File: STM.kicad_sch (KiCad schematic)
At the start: 25 parts, among them J7 PIN HEADER 2.54MM PITCH STR D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, U1 STM32L433CCU6

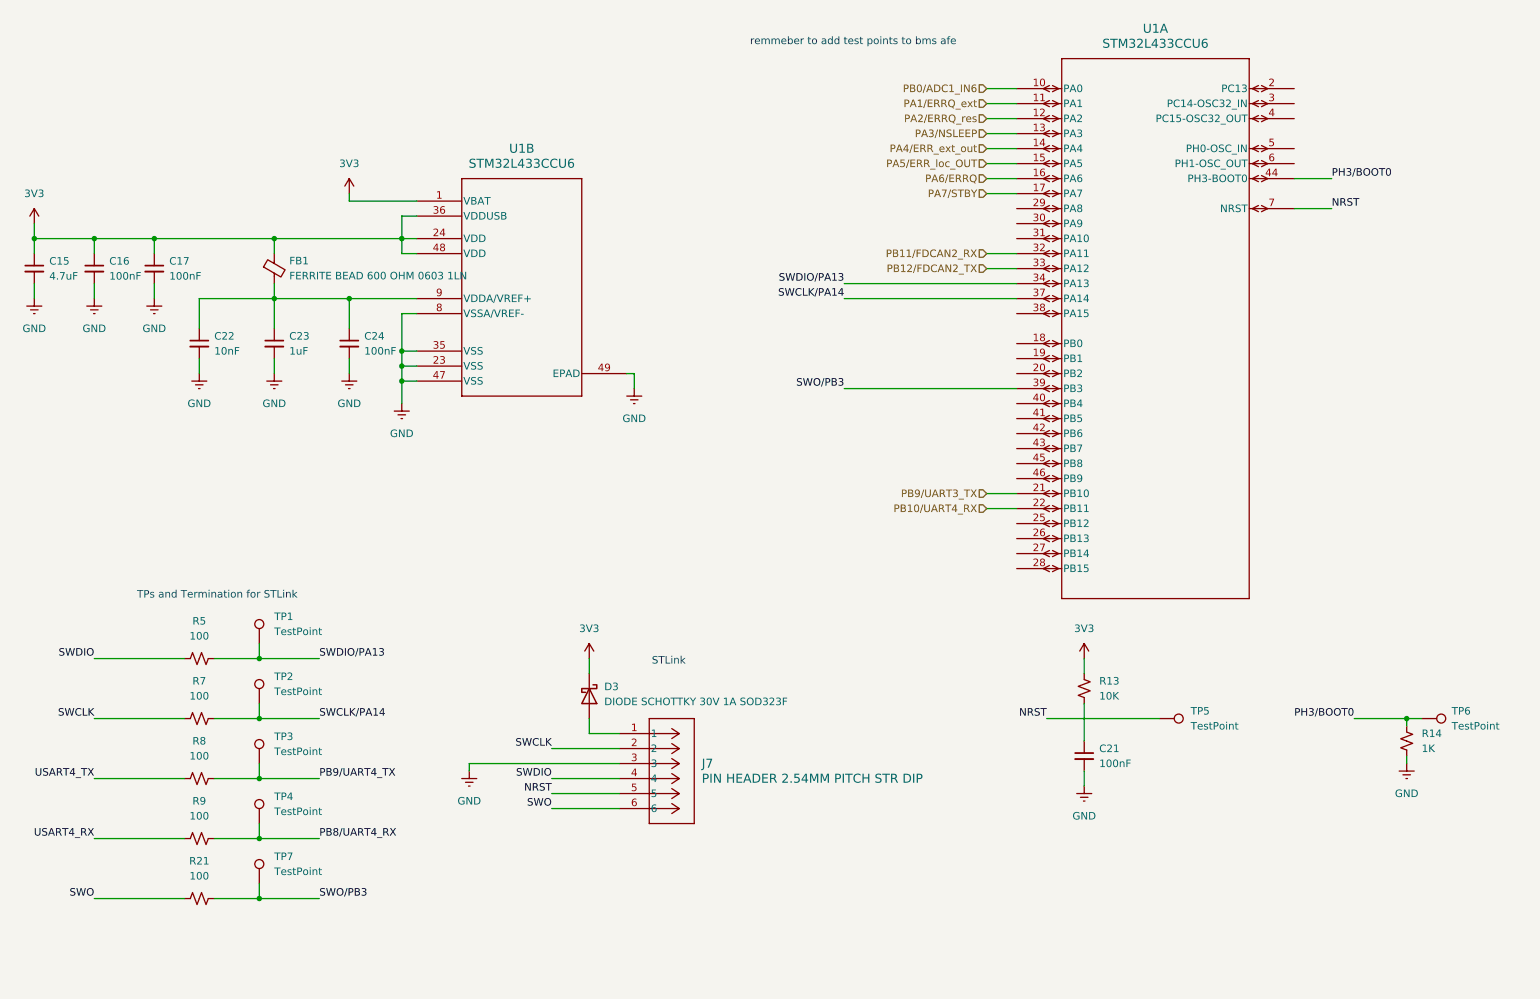
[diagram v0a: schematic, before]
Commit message: tweaked a little
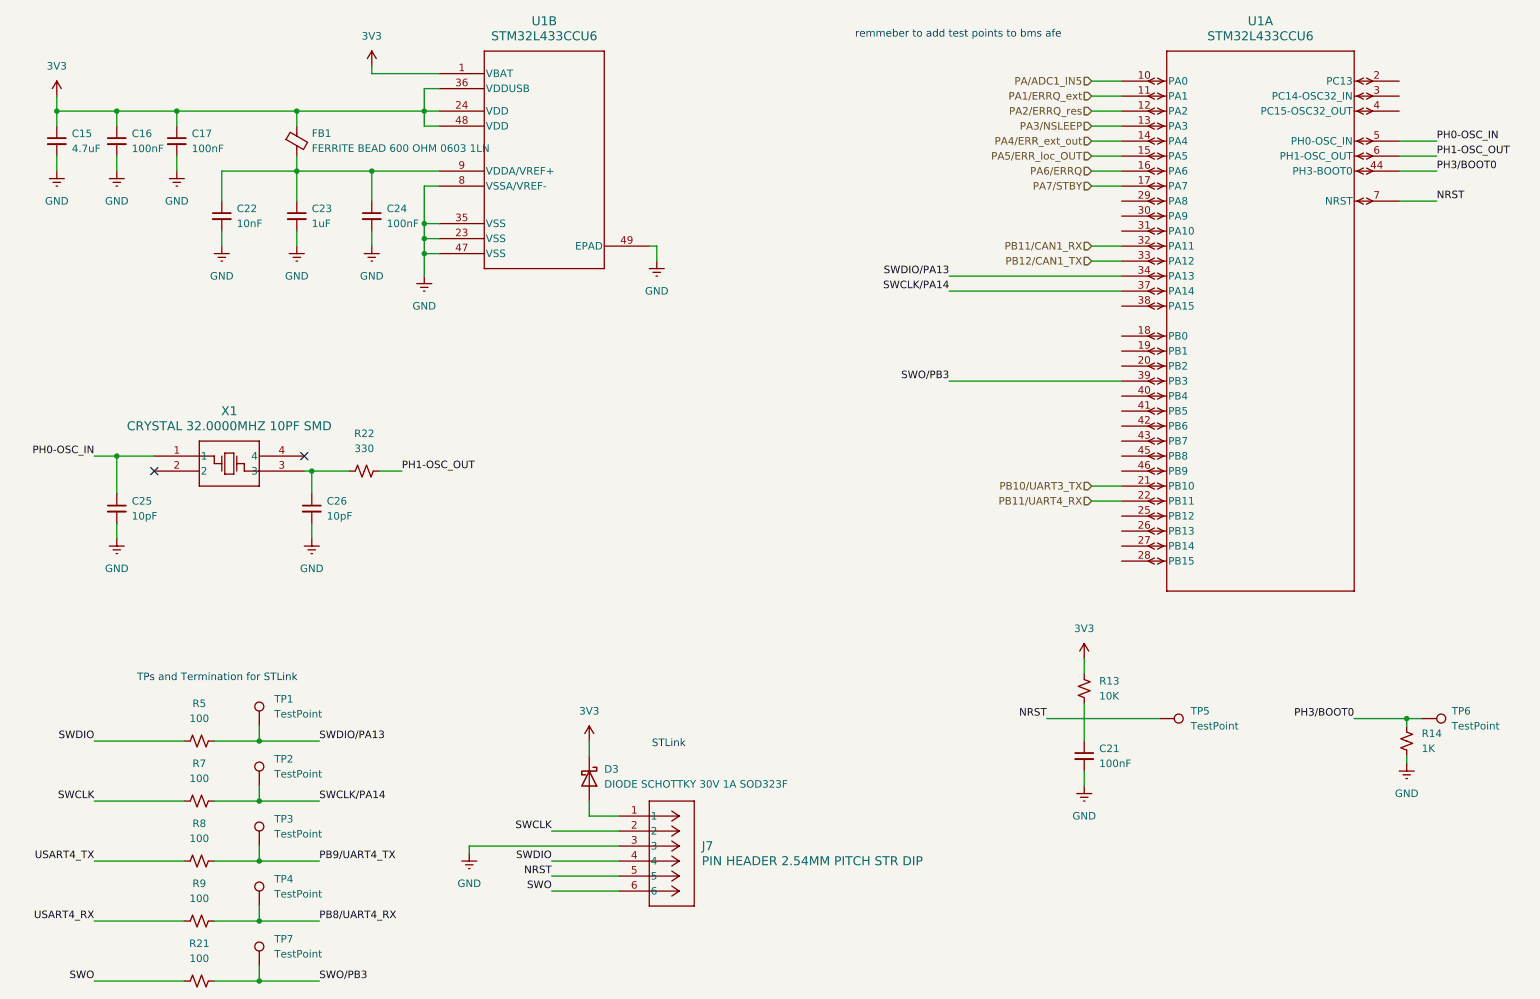
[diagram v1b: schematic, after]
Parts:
- added C25, C26: 10pF, symbol Device:C_Small
- added R22: 330, symbol Device:R_Small_US
- added X1: CRYSTAL 32.0000MHZ 10PF SMD, footprints:SMD4_RH100_2P5X3P2-2P2_RAL, symbol symbols:RH100-32.000-10-F-2020-EXT-TR
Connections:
- net GND: now also C25.2, C26.2
- net PH0-OSC_IN: now reaches U1.5 (PH0-OSC_IN)
- net PH0-OSC_IN: now also C25.1, X1.1
- net PH1-OSC_OUT: now reaches U1.6 (PH1-OSC_OUT)
- net PH1-OSC_OUT: now also R22.1
- net PB0/ADC1_IN6 renamed PA/ADC1_IN5
- net PB10/UART4_RX renamed PB11/UART4_RX
- net PB11/FDCAN2_RX renamed PB11/CAN1_RX
- net PB12/FDCAN2_TX renamed PB12/CAN1_TX
- net PB9/UART3_TX renamed PB10/UART3_TX
- new net: C26.1, R22.2, X1.3
- no-connect marks 0 -> 2
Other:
- moved on the sheet: C15, C16, C17, C22, C23, C24, D3, FB1, J7, R21, R5, R7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
